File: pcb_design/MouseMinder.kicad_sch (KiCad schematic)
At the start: 22 parts, among them J1 Conn_02x04_Odd_Even, Q1 SSM6L61NU,LF, SW1 SW_Push_Shielded, SW2 SW_Push_Shielded, U1 ATtiny10-TS

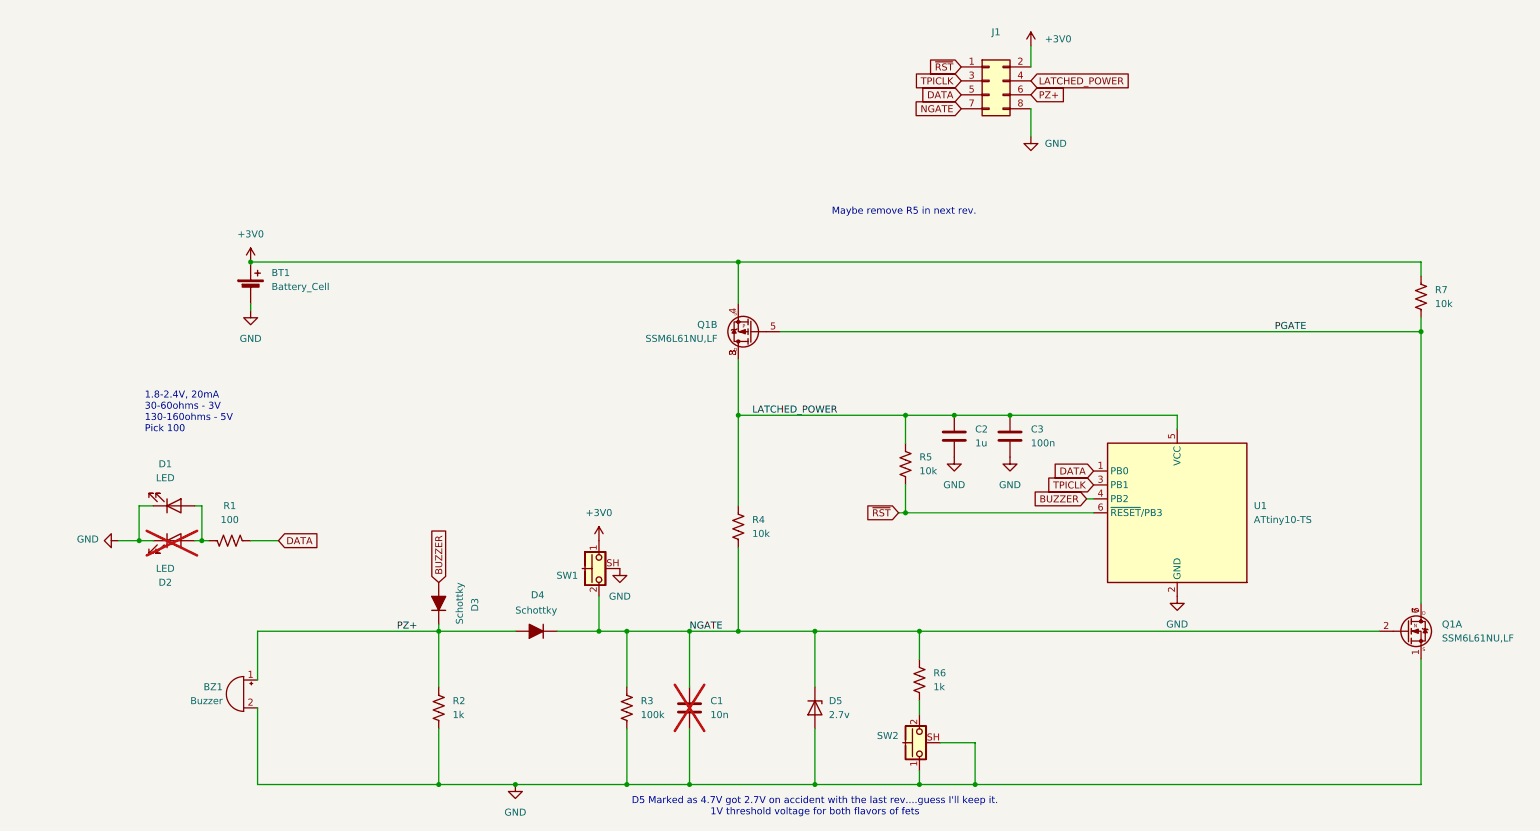
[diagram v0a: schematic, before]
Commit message: Latest and cost-optimized!
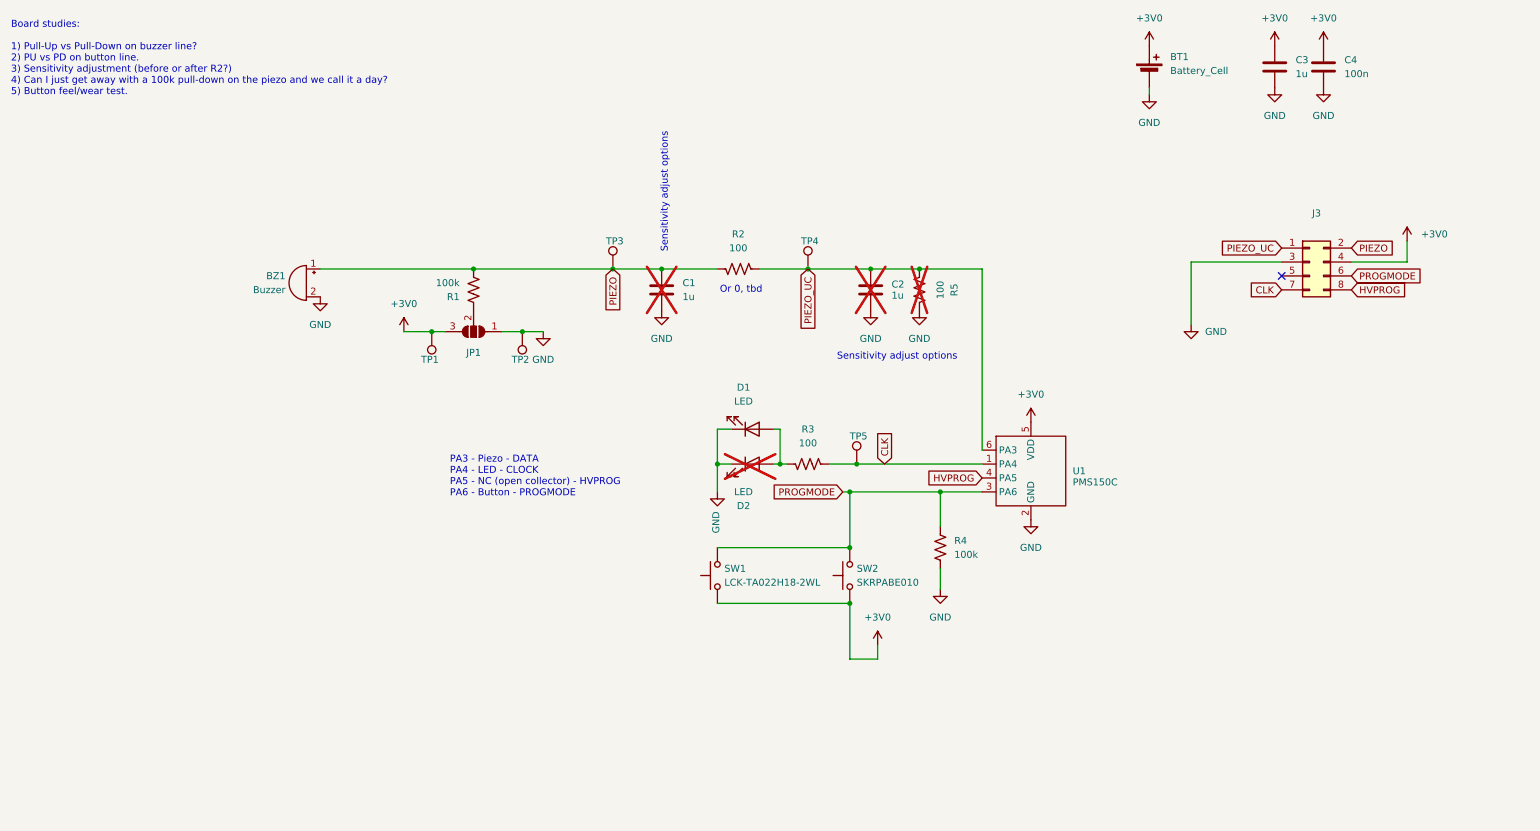
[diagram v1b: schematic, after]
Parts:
- removed D3, D4: Schottky, Diode_SMD:D_0603_1608Metric, symbol Device:D_Filled
- removed D5: 2.7v, Diode_SMD:D_0603_1608Metric, symbol Device:D_Zener
- removed Q1: SSM6L61NU,LF, 0conrads:SON65P200X200X80-8N, symbol 0conrads:SSM6L61NU,LF
- removed R3: 100k, Resistor_SMD:R_0402_1005Metric, symbol Device:R_US
- removed R6: 1k, Resistor_SMD:R_0402_1005Metric, symbol Device:R_US
- removed R7: 10k, Resistor_SMD:R_0402_1005Metric, symbol Device:R_US
- removed SW1, SW2: SW_Push_Shielded, Button_Switch_SMD:SW_Push_1P1T-SH_NO_CK_KMR2xxG, symbol Switch:SW_Push_Shielded
- removed U1: ATtiny10-TS, Package_TO_SOT_SMD:SOT-23-6, symbol MCU_Microchip_ATtiny:ATtiny10-TS
- added C4: 100n, Capacitor_SMD:C_0805_2012Metric, symbol Device:C
- added JP1: SolderJumper_3_Open, Jumper:SolderJumper-3_P1.3mm_Open_RoundedPad1.0x1.5mm_NumberLabels, symbol Jumper:SolderJumper_3_Open
- added R1: 100k, Resistor_SMD:R_0805_2012Metric, symbol Device:R_US
- added SW1: LCK-TA022H18-2WL, Button_Switch_SMD:SW_Push_1P1T_XKB_TS-1187A, symbol Switch:SW_Push
- added SW2: SKRPABE010, 0conrads:SKRPABE010, symbol Switch:SW_Push
- added TP1, TP2, TP3, TP4, TP5: TestPoint, TestPoint:TestPoint_Loop_D2.50mm_Drill1.0mm, symbol Connector:TestPoint
- added U1: PMS150C, Package_TO_SOT_SMD:SOT-23-6, symbol 0conrads:PMS150C
- BT1: footprint 0conrads:MY-2032-08 -> 0conrads:C70373; JLC_MPN C964831 -> C70373; MPN MY-2032-08 -> CR2032 3V
- C1: value 10n -> 1u; footprint Capacitor_SMD:C_0402_1005Metric -> Capacitor_SMD:C_0805_2012Metric
- C2: footprint Capacitor_SMD:C_0402_1005Metric -> Capacitor_SMD:C_0805_2012Metric; JLC_MPN C14445 -> (none); MPN CL05A105KP5NNNC -> (none); now not fitted; now left out of the parts list
- C3: value 100n -> 1u; footprint Capacitor_SMD:C_0402_1005Metric -> Capacitor_SMD:C_0805_2012Metric; JLC_MPN C1581 -> (none); MPN 0402F104M500NT -> (none)
- R2: value 1k -> 100; footprint Resistor_SMD:R_0402_1005Metric -> Resistor_SMD:R_0805_2012Metric; JLC_MPN C11702 -> C25076; MPN 0402WGF1001TCE -> 0402WGF1000TCE
- R3: renamed from R1; footprint Resistor_SMD:R_0402_1005Metric -> Resistor_SMD:R_0805_2012Metric
- R4: value 10k -> 100k; footprint Resistor_SMD:R_0402_1005Metric -> Resistor_SMD:R_0805_2012Metric; JLC_MPN C22356213 -> C25741; MPN RCA0210KJLF -> 0402WGF1003TCE
- R5: value 10k -> 100; footprint Resistor_SMD:R_0402_1005Metric -> Resistor_SMD:R_0805_2012Metric; JLC_MPN C22356213 -> C25076; MPN RCA0210KJLF -> 0402WGF1000TCE; now not fitted
- renumbered J1 to J3
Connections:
- net TPICLK is gone; now on net GND: J3.3 (Pin_3)
- net +3V0: now also C3.1, J3.4 (Pin_4), C4.1, JP1.3 (B), SW1.1, SW2.1, TP1.1, U1.5 (VDD); no longer J3.2 (Pin_2)
- net GND: now also R4.2, R5.1, C4.2, JP1.1 (A), TP2.1, U1.2 (GND); no longer J3.8 (Pin_8), R2.2
- net DATA: no longer names the net of J3.5 (Pin_5)
- net DATA: no longer R3.1
- removed net LATCHED_POWER: C2.1, C3.1, J3.4 (Pin_4), R4.1, R5.1
- removed net NGATE: C1.1, J3.7 (Pin_7), R4.2
- removed net PZ+: BZ1.1 (+), J3.6 (Pin_6), R2.1
- net ~{RST} renamed PIEZO_UC
- net PIEZO_UC: now also C2.1, R2.1, TP4.1, U1.6 (PA3)
- new net: JP1.2 (C), R1.1
- new net CLK: J3.7 (Pin_7), R3.1, TP5.1, U1.1 (PA4)
- new net HVPROG: J3.8 (Pin_8), U1.4 (PA5)
- new net PIEZO: BZ1.1 (+), C1.1, J3.2 (Pin_2), R1.2, R2.2, TP3.1
- new net PROGMODE: J3.6 (Pin_6), R4.1, SW1.2, SW2.2, U1.3 (PA6)
- no-connect marks 0 -> 1
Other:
- note added: "Board studies: 1) Pull-Up vs Pull-Down on buzzer line? 2) PU vs PD on button line. 3) Sensitivity adjustment (before or after R2?) 4) Can I just get away with a 100k pull-down on the piezo and we call it a day? 5) Button feel/wear test."
- note added: "Or 0, tbd"
- note added: "PA3 - Piezo - DATA PA4 - LED - CLOCK PA5 - NC (open collector) - HVPROG PA6 - Button - PROGMODE"
- note added: "Sensitivity adjust options"
- note removed: "1.8-2.4V, 20mA 30-60ohms - 3V 130-160ohms - 5V Pick 100"
- note removed: "D5 Marked as 4.7V got 2.7V on accident with the last rev....guess I'll keep it. 1V threshold voltage for both flavors of fets"
- note removed: "Maybe remove R5 in next rev."
- moved on the sheet: BZ1, D1, D2, J3, R3
